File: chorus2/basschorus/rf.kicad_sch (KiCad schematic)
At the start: 11 parts, among them U2 TL074

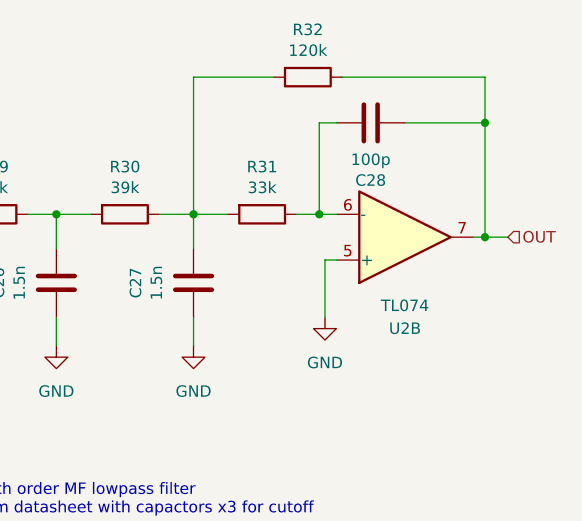
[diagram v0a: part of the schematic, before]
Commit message: basic layout
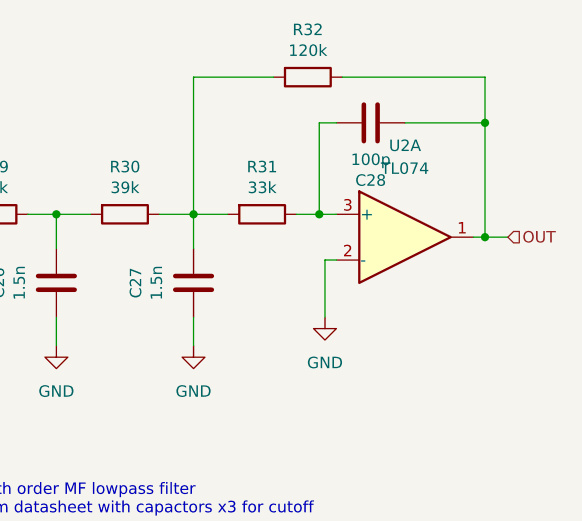
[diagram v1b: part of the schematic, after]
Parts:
- removed U2: TL074, Package_SO:SO-14_3.9x8.65mm_P1.27mm, symbol Amplifier_Operational:TL074
- added U2: TL074, Package_SO:SO-14_3.9x8.65mm_P1.27mm, symbol Amplifier_Operational:TL074
- R28, R29, R30, R31, R32: footprint Resistor_THT:R_Axial_DIN0204_L3.6mm_D1.6mm_P5.08mm_Horizontal -> Resistor_THT:R_Axial_DIN0204_L3.6mm_D1.6mm_P2.54mm_Vertical
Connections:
- net GND: now also U2.2 (-)
- net OUT: now also U2.1
- net at C28.1, R31.1: now also U2.3 (+)
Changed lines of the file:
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@@
 			)
 		)
-		(property "Footprint" "Resistor_THT:R_Axial_DIN0204_L3.6mm_D1.6mm_P5.08mm_Horizontal"
+		(property "Footprint" "Resistor_THT:R_Axial_DIN0204_L3.6mm_D1.6mm_P2.54mm_Vertical"
 			(at 141.605 80.137 90)
 			(effects
@@
 			)
 		)
-		(property "Footprint" "Resistor_THT:R_Axial_DIN0204_L3.6mm_D1.6mm_P5.08mm_Horizontal"
+		(property "Footprint" "Resistor_THT:R_Axial_DIN0204_L3.6mm_D1.6mm_P2.54mm_Vertical"
 			(at 127.635 80.137 90)
 			(effects
@@
 	)
 	(symbol
+		(lib_id "Amplifier_Operational:TL074")
+		(at 187.325 84.455 0)
+		(unit 1)
+		(exclude_from_sim no)
+		(in_bom yes)
+		(on_board yes)
+		(dnp no)
+		(fields_autoplaced yes)
+		(property "Reference" "U2"
+			(at 187.325 74.295 0)
+			(effects
+				(font
+					(size 1.27 1.27)
+				)
+			)
+		)
+		(property "Value" "TL074"
+			(at 187.325 76.835 0)
+			(effects
+				(font
+					(size 1.27 1.27)
+				)
+			)
+		)
+		(property "Footprint" "Package_SO:SO-14_3.9x8.65mm_P1.27mm"
+			(at 186.055 81.915 0)
+			(effects
+				(font
+					(size 1.27 1.27)
+				)
+				(hide yes)
+			)
+		)
+		(property "Datasheet" "http://www.ti.com/lit/ds/symlink/tl071.pdf"
+			(at 188.595 79.375 0)
+			(effects
+				(font
+					(size 1.27 1.27)
+				)
+				(hide yes)
+			)
+		)
+		(property "Description" "Quad Low-Noise JFET-Input Operational Amplifiers, DIP-14/SOIC-14"
+			(at 187.325 84.455 0)
+			(effects
+				(font
+					(size 1.27 1.27)
+				)
+				(hide yes)
+			)
+		)
+		(pin "1"
+		)
+		(pin "5"
+		)
+		(pin "3"
+		)
+		(pin "2"
+		)
+		(pin "6"
+		)
+		(pin "7"
+		)
+		(pin "10"
+		)
+		(pin "9"
+		)
+		(pin "8"
+		)
+		(pin "12"
+		)
+		(pin "13"
+		)
+		(pin "4"
+		)
+		(pin "11"
+		)
+		(pin "14"
+		)
+		(instances
+			(project "basschorus"
+				(path "/7f3b4bac-3b2a-4af0-92ae-ccc3fcedc393/89406d17-d719-4016-b0cb-a2835ffb8d3f"
+					(reference "U2")
+					(unit 1)
+				)
+			)
+		)
+	)
+	(symbol
 		(lib_id "power:GND")
 		(at 163.83 96.52 0)
@@
 			)
 		)
-		(property "Footprint" "Resistor_THT:R_Axial_DIN0204_L3.6mm_D1.6mm_P5.08mm_Horizontal"
+		(property "Footprint" "Resistor_THT:R_Axial_DIN0204_L3.6mm_D1.6mm_P2.54mm_Vertical"
 			(at 171.45 80.137 90)
 			(effects
@@
 	)
 	(symbol
-		(lib_id "Amplifier_Operational:TL074")
-		(at 187.325 84.455 0)
-		(mirror x)
-		(unit 2)
-		(exclude_from_sim no)
-		(in_bom yes)
-		(on_board yes)
-		(dnp no)
-		(property "Reference" "U2"
-			(at 187.325 94.615 0)
-			(effects
-				(font
-					(size 1.27 1.27)
-				)
-			)
-		)
-		(property "Value" "TL074"
-			(at 187.325 92.075 0)
-			(effects
-				(font
-					(size 1.27 1.27)
-				)
-			)
-		)
-		(property "Footprint" "Package_SO:SO-14_3.9x8.65mm_P1.27mm"
-			(at 186.055 86.995 0)
-			(effects
-				(font
-					(size 1.27 1.27)
-				)
-				(hide yes)
-			)
-		)
-		(property "Datasheet" "http://www.ti.com/lit/ds/symlink/tl071.pdf"
-			(at 188.595 89.535 0)
-			(effects
-				(font
-					(size 1.27 1.27)
-				)
-				(hide yes)
-			)
-		)
-		(property "Description" "Quad Low-Noise JFET-Input Operational Amplifiers, DIP-14/SOIC-14"
-			(at 187.325 84.455 0)
-			(effects
-				(font
-					(size 1.27 1.27)
-				)
-				(hide yes)
-			)
-		)
-		(pin "1"
-		)
-		(pin "3"
-		)
-		(pin "2"
-		)
-		(pin "5"
-		)
-		(pin "14"
-		)
-		(pin "10"
-		)
-		(pin "8"
-		)
-		(pin "6"
-		)
-		(pin "9"
-		)
-		(pin "11"
-		)
-		(pin "12"
-		)
-		(pin "7"
-		)
-		(pin "13"
-		)
-		(pin "4"
-		)
-		(instances
-			(project "basschorus"
-				(path "/7f3b4bac-3b2a-4af0-92ae-ccc3fcedc393/89406d17-d719-4016-b0cb-a2835ffb8d3f"
-					(reference "U2")
-					(unit 2)
-				)
-			)
-		)
-	)
-	(symbol
 		(lib_id "Device:R")
 		(at 156.21 81.915 270)
@@
 			)
 		)
-		(property "Footprint" "Resistor_THT:R_Axial_DIN0204_L3.6mm_D1.6mm_P5.08mm_Horizontal"
+		(property "Footprint" "Resistor_THT:R_Axial_DIN0204_L3.6mm_D1.6mm_P2.54mm_Vertical"
 			(at 156.21 80.137 90)
 			(effects
@@
 			)
 		)
-		(property "Footprint" "Resistor_THT:R_Axial_DIN0204_L3.6mm_D1.6mm_P5.08mm_Horizontal"
+		(property "Footprint" "Resistor_THT:R_Axial_DIN0204_L3.6mm_D1.6mm_P2.54mm_Vertical"
 			(at 176.53 64.897 90)
 			(effects
